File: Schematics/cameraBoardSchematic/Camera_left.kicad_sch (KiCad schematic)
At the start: 7 parts, among them IC1 LM3940IS-3.3_NOPB

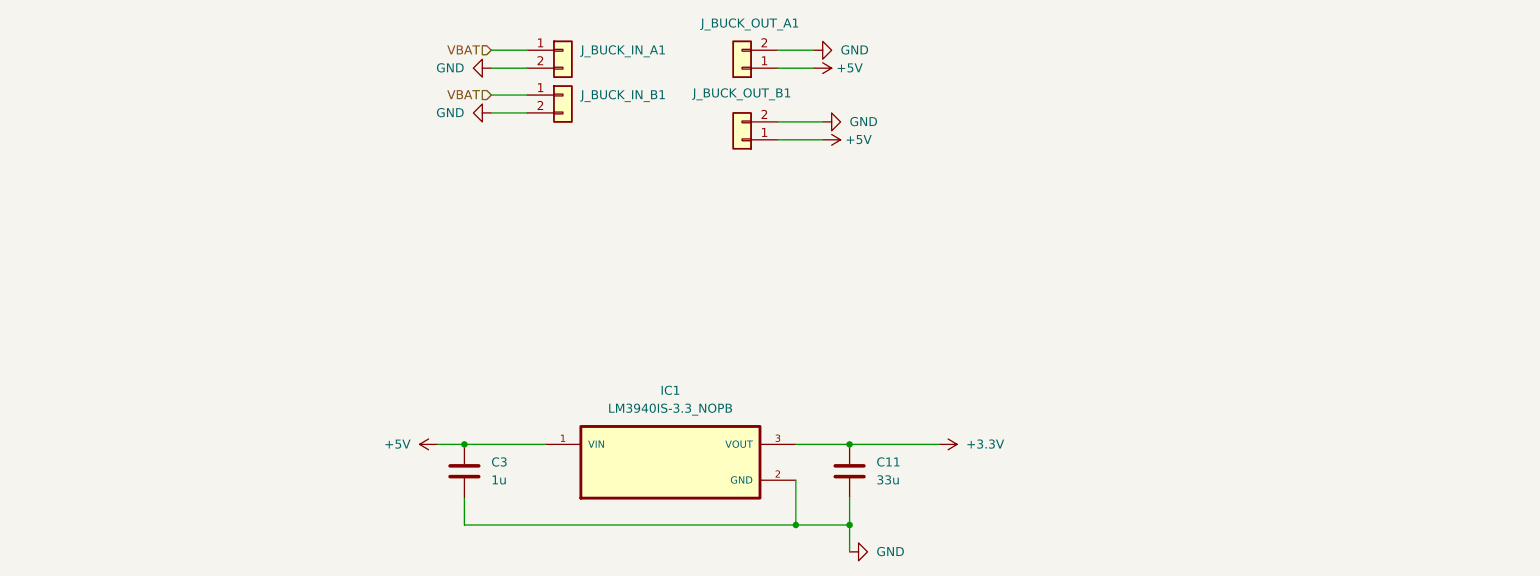
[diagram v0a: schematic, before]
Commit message: first PCB Draft
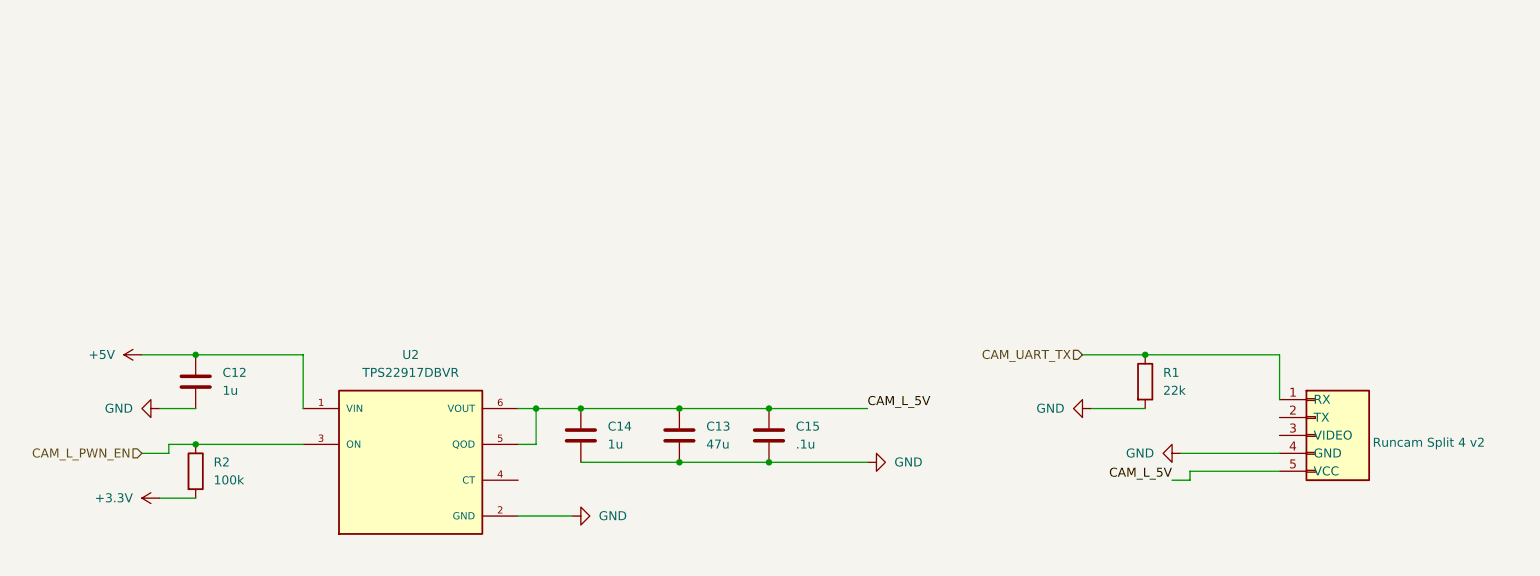
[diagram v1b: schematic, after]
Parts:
- removed C11: 33u, Capacitor_SMD:C_0805_2012Metric_Pad1.18x1.45mm_HandSolder, symbol Device:C
- removed C3: 1u, Capacitor_SMD:C_0805_2012Metric_Pad1.18x1.45mm_HandSolder, symbol Device:C
- removed IC1: LM3940IS-3.3_NOPB, myFootprints:TO254P1524X483-4N, symbol LM3940IS-3.3_NOPB:LM3940IS-3.3_NOPB
- removed J_BUCK_IN_A1, J_BUCK_IN_B1, J_BUCK_OUT_A1, J_BUCK_OUT_B1: ~, Capacitor_SMD:C_0805_2012Metric_Pad1.18x1.45mm_HandSolder, symbol Connector_Generic:Conn_01x02
- added C12, C14: 1u, Capacitor_SMD:C_0805_2012Metric_Pad1.18x1.45mm_HandSolder, symbol Device:C
- added C13: 47u, Capacitor_SMD:C_0805_2012Metric_Pad1.18x1.45mm_HandSolder, symbol Device:C
- added C15: .1u, Capacitor_SMD:C_0805_2012Metric_Pad1.18x1.45mm_HandSolder, symbol Device:C
- added J1: Runcam Split 4 v2, Capacitor_SMD:C_0805_2012Metric_Pad1.18x1.45mm_HandSolder, symbol Connector_Generic:Conn_01x05
- added R1: 22k, Resistor_SMD:R_0805_2012Metric_Pad1.20x1.40mm_HandSolder, symbol Device:R
- added R2: 100k, Resistor_SMD:R_0805_2012Metric_Pad1.20x1.40mm_HandSolder, symbol Device:R
- added U2: TPS22917DBVR, myFootprints:SOT95P280X145-6N, symbol TPS22917DBVR:TPS22917DBVR
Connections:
- net +3.3V: now also R2.2
- net +5V: now also C12.1, U2.1 (VIN)
- net GND: now also C12.2, C13.2, C14.2, C15.2, J1.4 (GND), R1.2, U2.2 (GND)
- new net: C13.1, C14.1, C15.1, J1.5 (VCC), U2.5 (QOD), U2.6 (VOUT)
- new net CAM_L_PWN_EN: R2.1, U2.3 (ON)
- new net CAM_UART_TX: J1.1 (RX), R1.1
